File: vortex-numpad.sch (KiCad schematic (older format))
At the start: 60 parts, among them J1 USB_B_Micro, SW1 SW_Push, U1 ATmega32U4-AU, Y1 16MHz

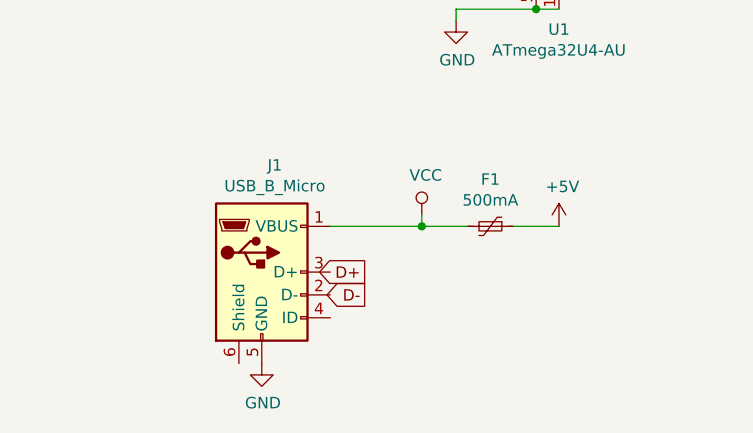
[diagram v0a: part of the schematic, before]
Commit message: Initial PCB layout
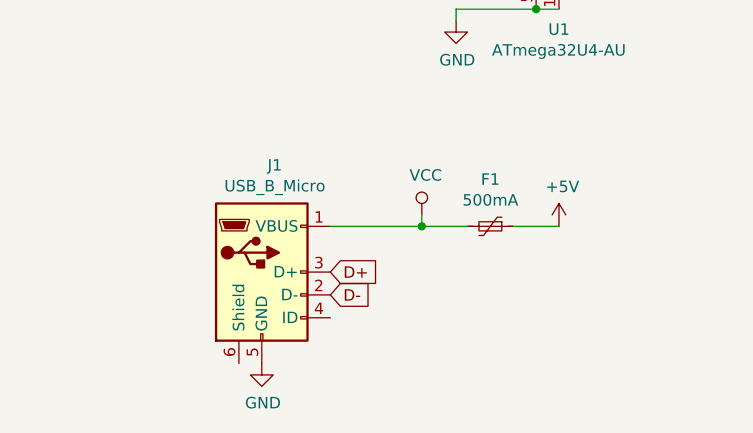
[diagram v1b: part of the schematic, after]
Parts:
- PLUS1, RETURN1: footprint MX_Alps_Hybrid:MX-1U-NoLED -> MX_Alps_Hybrid:MX-2U-ReversedStabilizers-NoLED
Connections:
- net D+: now also J1.3 (D+)
- net D-: now also J1.2 (D-)
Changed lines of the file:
@@
 Wire Wire Line
 	3100 5900 2900 5900
-Text GLabel 2250 6200 0    50   Output ~ 0
+Text GLabel 2100 6200 2    50   Input ~ 0
 D-
-Text GLabel 2250 6100 0    50   Output ~ 0
+Text GLabel 2100 6100 2    50   Input ~ 0
 D+
 $Comp
@@
 F 0 "PLUS1" H 7083 3573 60  0000 C CNN
 F 1 "MX-NoLED" H 7083 3499 20  0000 C CNN
-F 2 "MX_Alps_Hybrid:MX-1U-NoLED" H 6425 3325 60  0001 C CNN
+F 2 "MX_Alps_Hybrid:MX-2U-ReversedStabilizers-NoLED" H 6425 3325 60  0001 C CNN
 F 3 "" H 6425 3325 60  0001 C CNN
 	1    7050 3350
@@
 F 0 "RETURN1" H 7083 4973 60  0000 C CNN
 F 1 "MX-NoLED" H 7083 4899 20  0000 C CNN
-F 2 "MX_Alps_Hybrid:MX-1U-NoLED" H 6425 4725 60  0001 C CNN
+F 2 "MX_Alps_Hybrid:MX-2U-ReversedStabilizers-NoLED" H 6425 4725 60  0001 C CNN
 F 3 "" H 6425 4725 60  0001 C CNN
 	1    7050 4750
